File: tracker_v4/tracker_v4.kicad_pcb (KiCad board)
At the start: 4 copper layers, 63.2 x 26 mm, 53 parts, among them IC1 RT9080-33GJ5, J1 USB_C_Receptacle_USB2.0_16P, Q1 DMG9926UDM-7, SW1 SW_Push, SW2 SW_Push, U1 ESP32-C6-MINI-1-N4, U2 LIS3DH, U3 DW01A, U4 INA226AIDGSR, U5 TP4056-42-ESOP8, U6 USBLC6-2SC6, U7 TPS3899DL01DSER

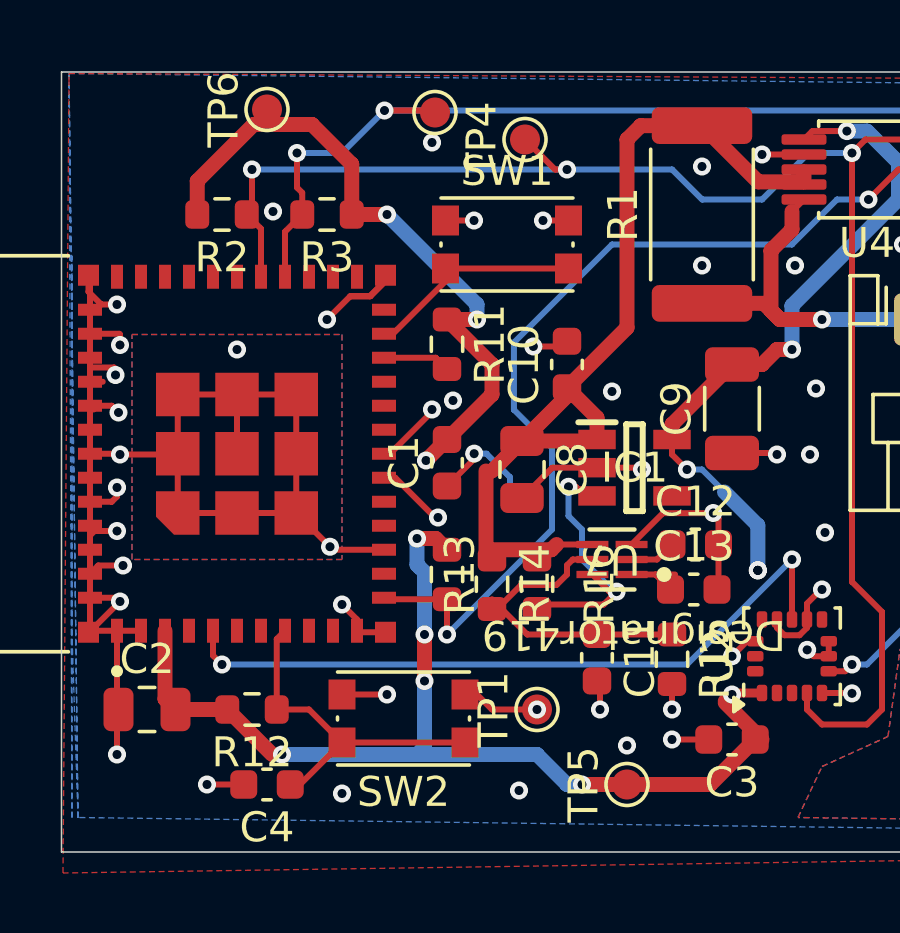
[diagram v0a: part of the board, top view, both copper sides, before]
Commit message: jkd
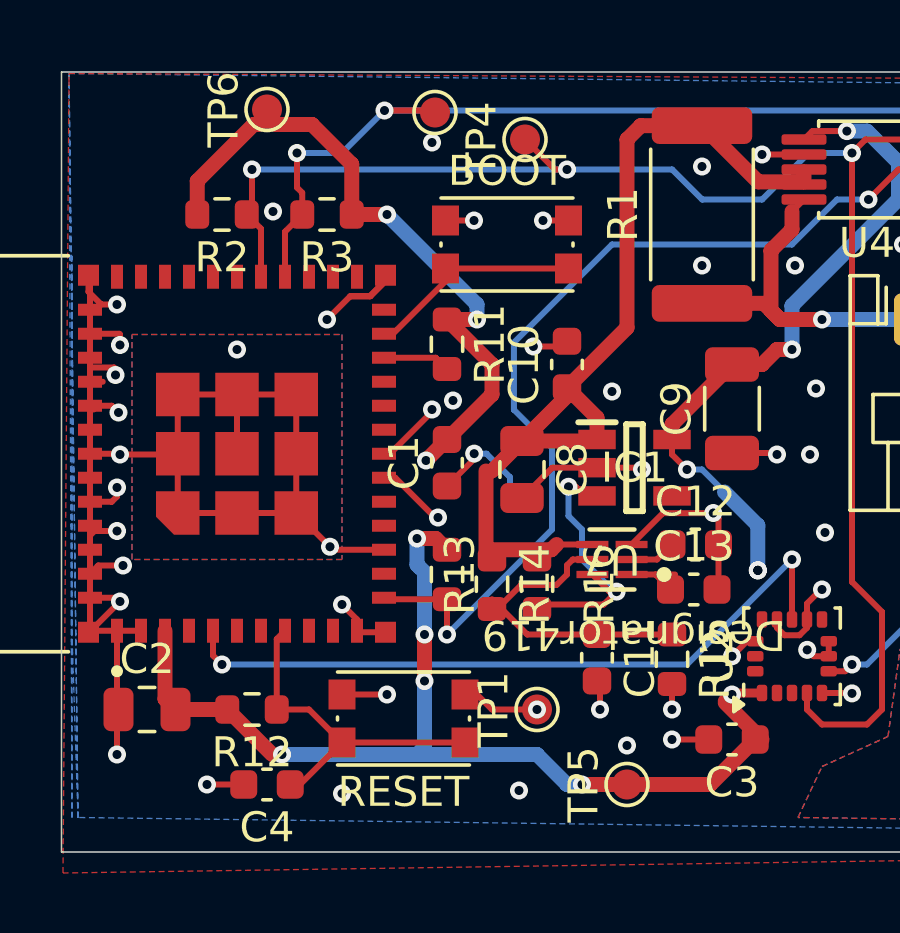
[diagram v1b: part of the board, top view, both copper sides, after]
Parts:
- renumbered SW1 to BOOT, SW2 to RESET
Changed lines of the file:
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@@
 		(capping no)
 		(filling no)
-		(zone_defaults)
 		(pcbplotparams
 			(layerselection 0x00000000_00000000_55555555_5755f5ff)
@@
 		(descr "CK components KMR2 tactile switch http://www.ckswitches.com/media/1479/kmr2.pdf")
 		(tags "tactile switch kmr2")
-		(property "Reference" "SW1"
+		(property "Reference" "BOOT"
 			(at 0 -2.45 0)
 			(layer "F.SilkS")
@@
 		(descr "CK components KMR2 tactile switch http://www.ckswitches.com/media/1479/kmr2.pdf")
 		(tags "tactile switch kmr2")
-		(property "Reference" "SW2"
+		(property "Reference" "RESET"
 			(at 0 -2.45 0)
 			(layer "F.SilkS")
